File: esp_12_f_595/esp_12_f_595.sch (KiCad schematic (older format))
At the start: 21 parts, among them P0 RGB_OUT, P1 RGB_OUT, P2 RGB_OUT, P3 CONN_01X04, P4 MicroB, SW1 TACTILE, U1 74HC595, U2 74HC595, U3 AP1117v3.3, U4 74HC595, U5 74HC595

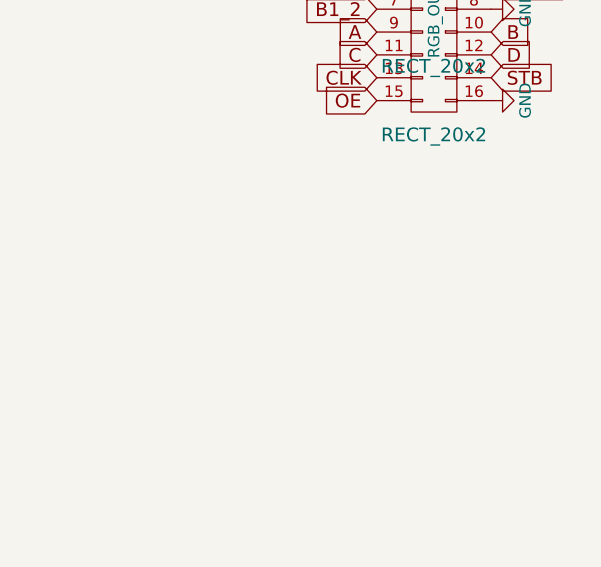
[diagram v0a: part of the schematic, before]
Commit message: Update design
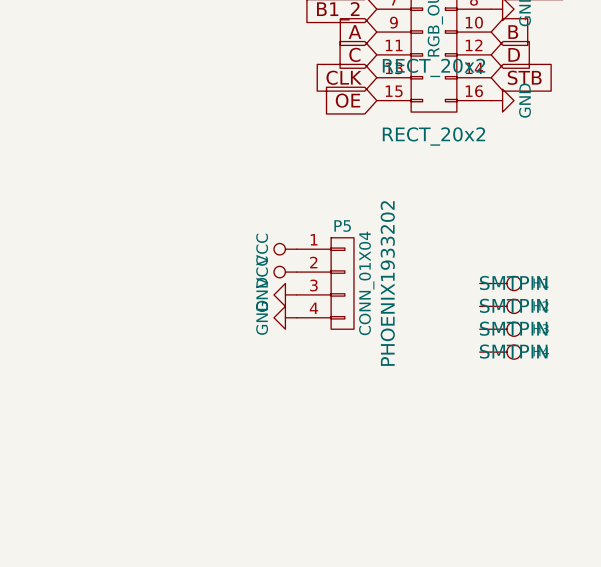
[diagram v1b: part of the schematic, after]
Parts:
- added H1, H2, H3, H4: MH, SMTPIN, symbol CONN_1
- added P5: CONN_01X04, PHOENIX1933202, symbol CONN_01X04
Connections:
- net +5V: now also P5.1 (P1), P5.2 (P2)
- net GND: now also P5.3 (P3), P5.4 (P4)
